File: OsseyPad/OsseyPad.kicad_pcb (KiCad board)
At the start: 4 copper layers, 152.4 x 142.9 mm, 96 parts, among them J1 USB_C_Receptacle_USB2.0, SW1 Rotary_Encoder_Switch, SW2 SW_Push, U1 USBLC6-2SC6, U2 ATmega32U4-MU, Y1 16MHz

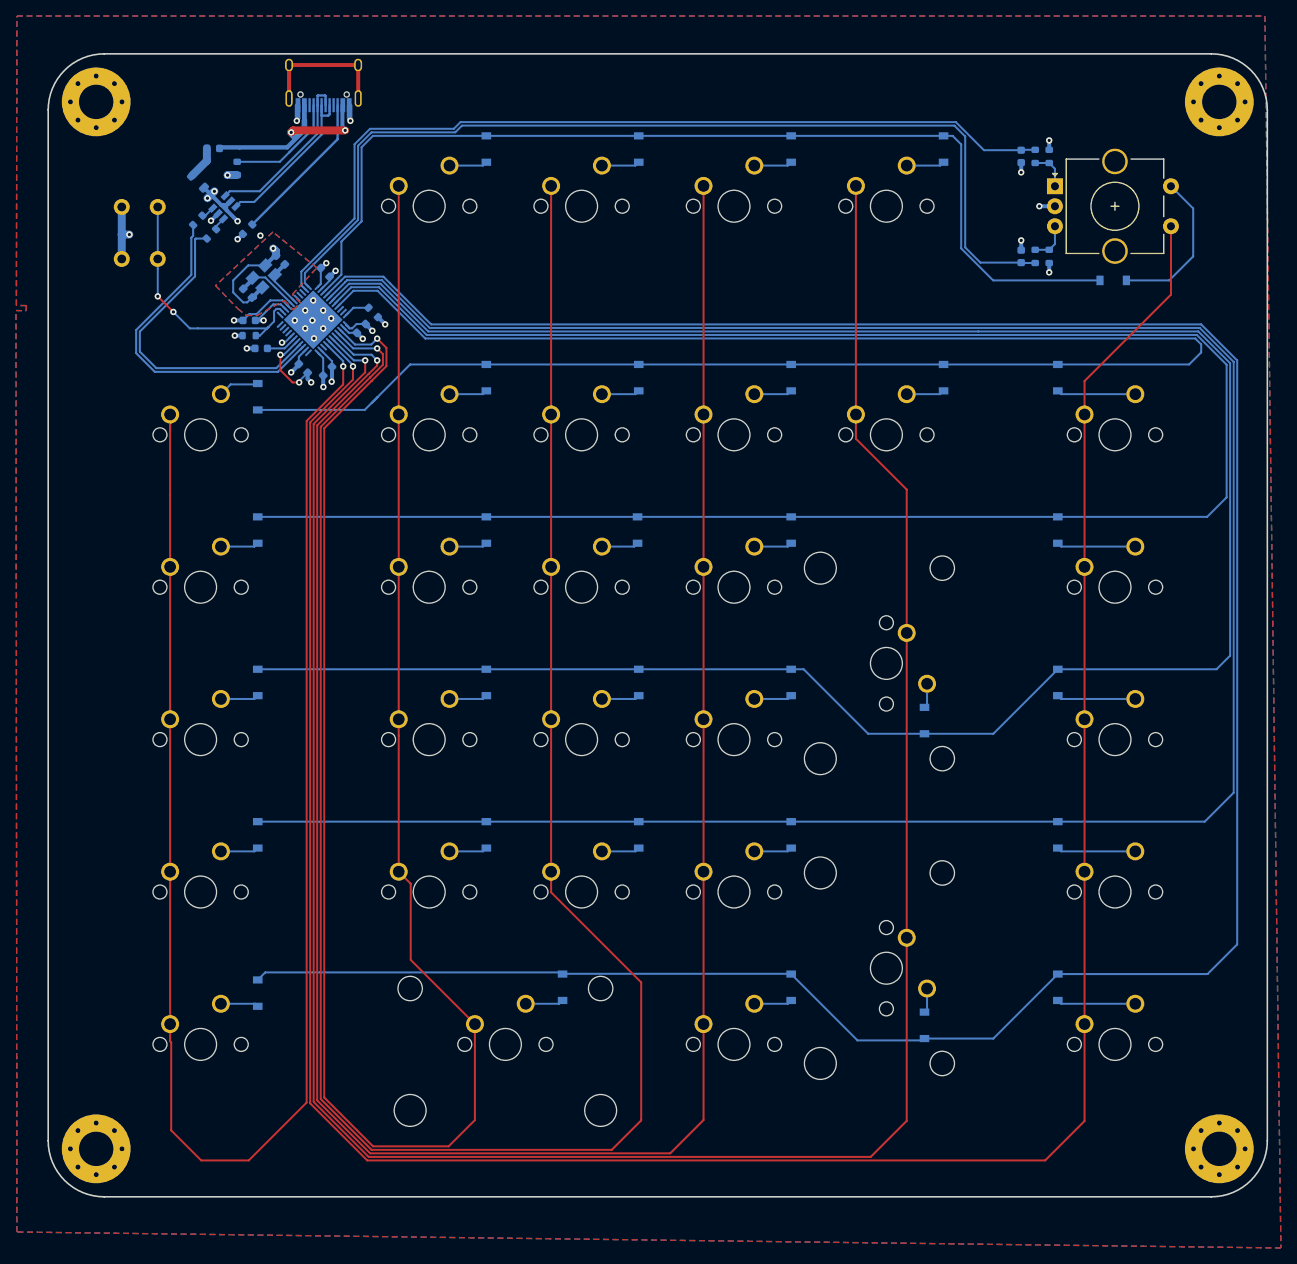
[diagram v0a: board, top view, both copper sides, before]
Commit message: PCB Update.
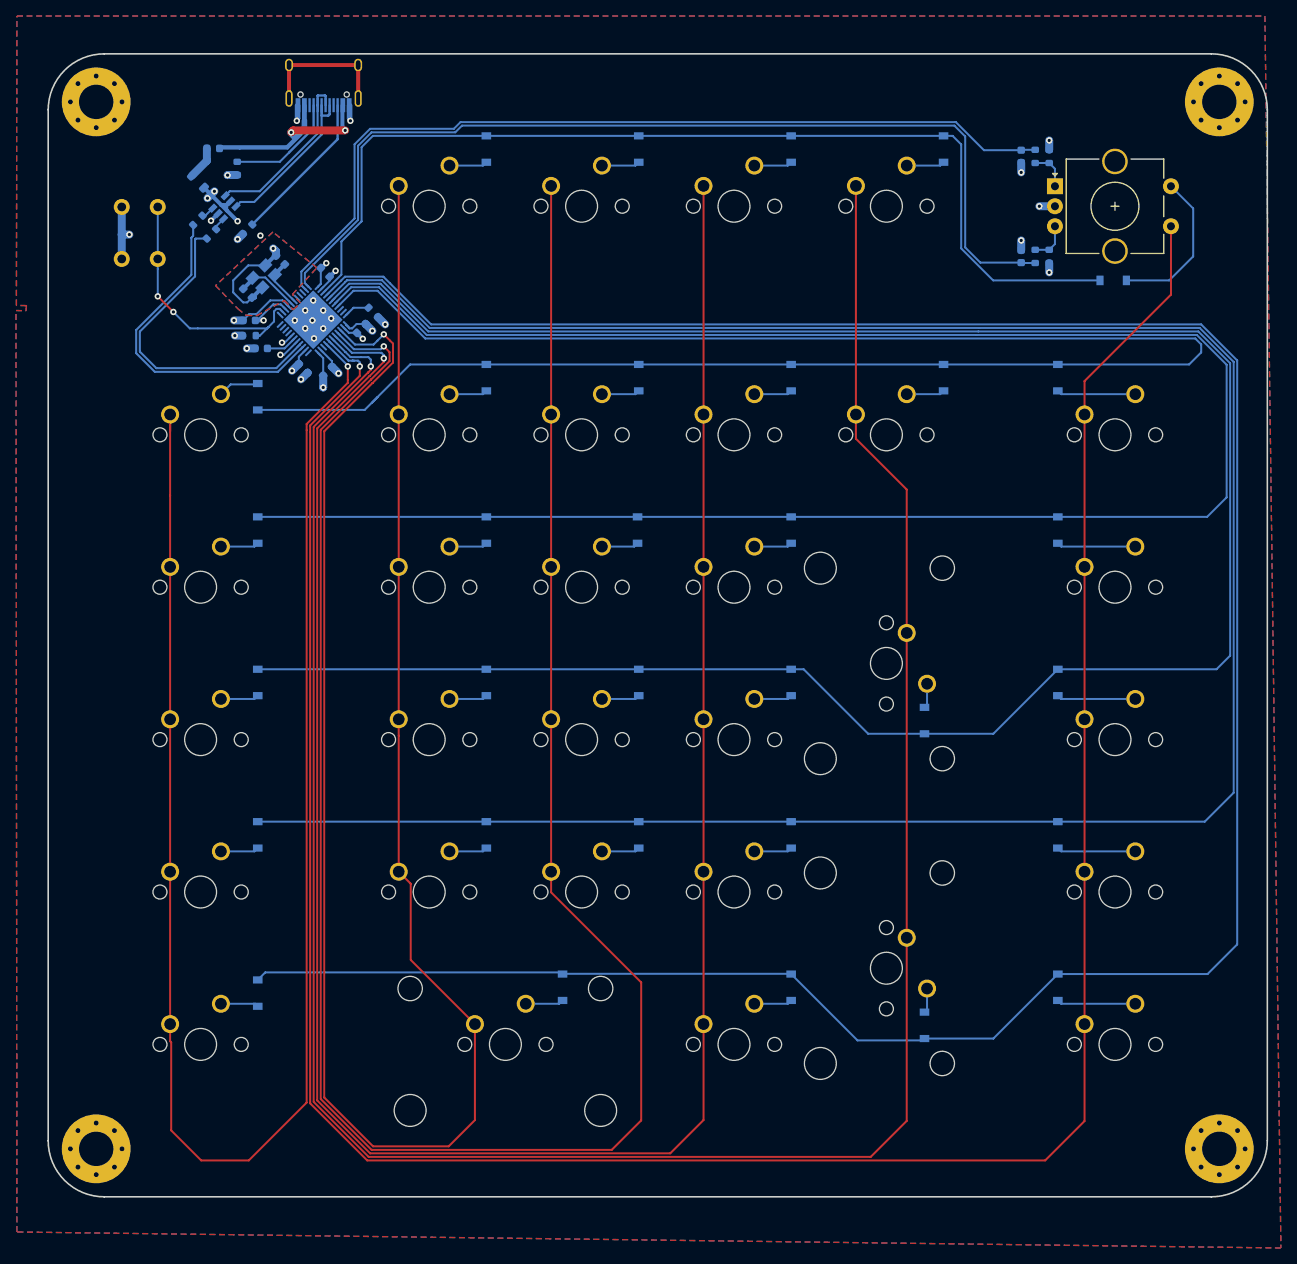
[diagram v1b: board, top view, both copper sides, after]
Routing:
- net GND: track 72.7 -> 65.2 mm, vias 29 -> 28
- net COL1: track 247.6 -> 249.6 mm
- net COL2: track 268.8 -> 270.4 mm
- net COL5: track 316.9 -> 318.5 mm
- net COL3: track 271.7 -> 273.3 mm
- net COL4: track 299.0 -> 300.2 mm
